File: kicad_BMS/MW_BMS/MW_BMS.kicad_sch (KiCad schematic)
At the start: 82 parts, among them J1 Conn_01x02_Pin, J3 Conn_01x05_Pin, J4 Conn_01x02_Pin, Q1 CSD17578Q5A, Q3 NPN_BSS306NH6327XTSA1, Q4 PNP_BSS308PE, Q5 NPN_BSS306NH6327XTSA1, Q6 PNP_BSS308PE, T1 Transformer_1P_1S, U1 L9963E-TR, U2 USBLC6-2SC6Y, U3 USBLC6-2SC6Y

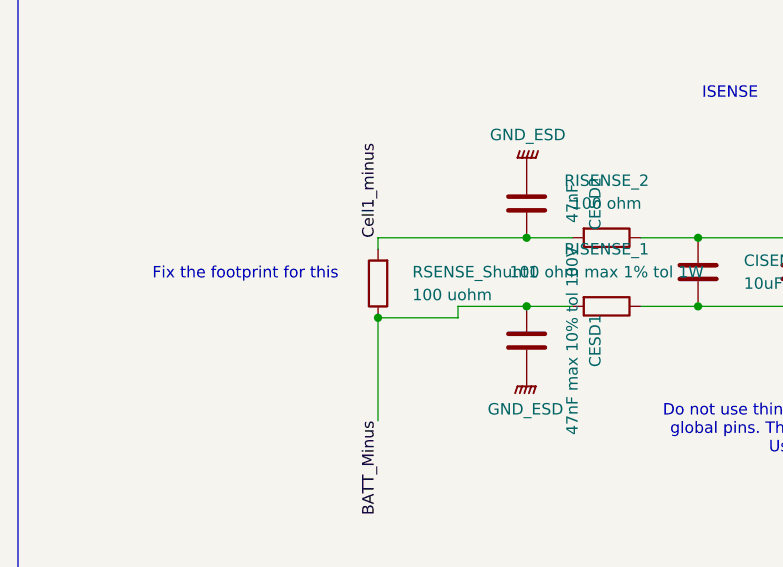
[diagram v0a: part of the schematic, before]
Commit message: most_routing_done
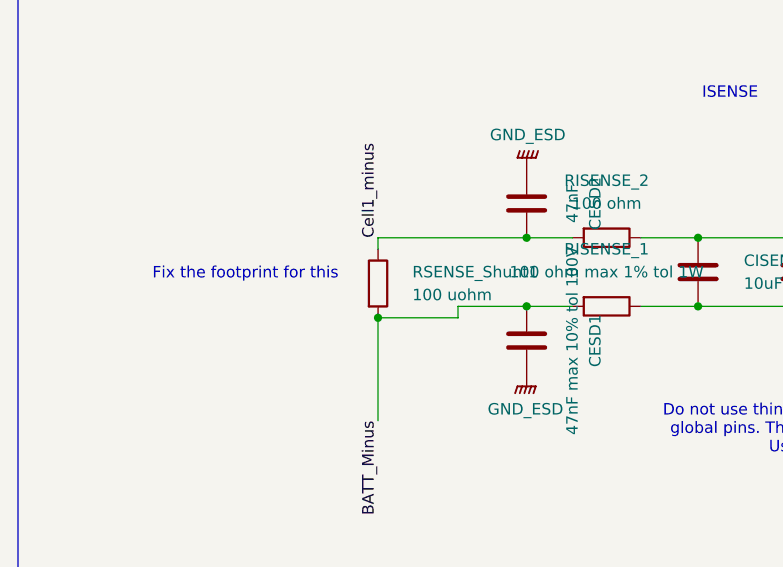
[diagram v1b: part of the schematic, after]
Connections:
- net BATT_Minus: now also RSENSE_Shunt1.2; no longer RSENSE_Shunt1.1
- net Cell1_minus: now also RSENSE_Shunt1.1; no longer RSENSE_Shunt1.2
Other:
- moved on the sheet: RSENSE_Shunt1
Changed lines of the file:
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@@
 	)
 	(junction
-		(at 144.78 64.77)
+		(at -97.79 157.48)
 		(diameter 0)
 		(color 0 0 0 0)
 	)
 	(junction
-		(at -97.79 157.48)
+		(at 144.78 64.77)
 		(diameter 0)
 		(color 0 0 0 0)
@@
 	(symbol
 		(lib_id "Device:R")
-		(at -97.79 153.67 180)
+		(at -97.79 153.67 0)
 		(unit 1)
 		(body_style 1)
@@
 					(size 1.27 1.27)
 				)
-				(justify right)
+				(justify left)
 			)
 		)
@@
 					(size 1.27 1.27)
 				)
-				(justify right)
+				(justify left)
 			)
 		)
 		(property "Footprint" "CSS2H-3920:Shunt"
-			(at -96.012 153.67 90)
+			(at -99.568 153.67 90)
 			(hide yes)
 			(show_name no)
